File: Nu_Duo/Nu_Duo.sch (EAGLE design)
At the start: 11 parts, among them P1 XR_PREAMP, P2 XR_PREAMP, SW1 TDS08

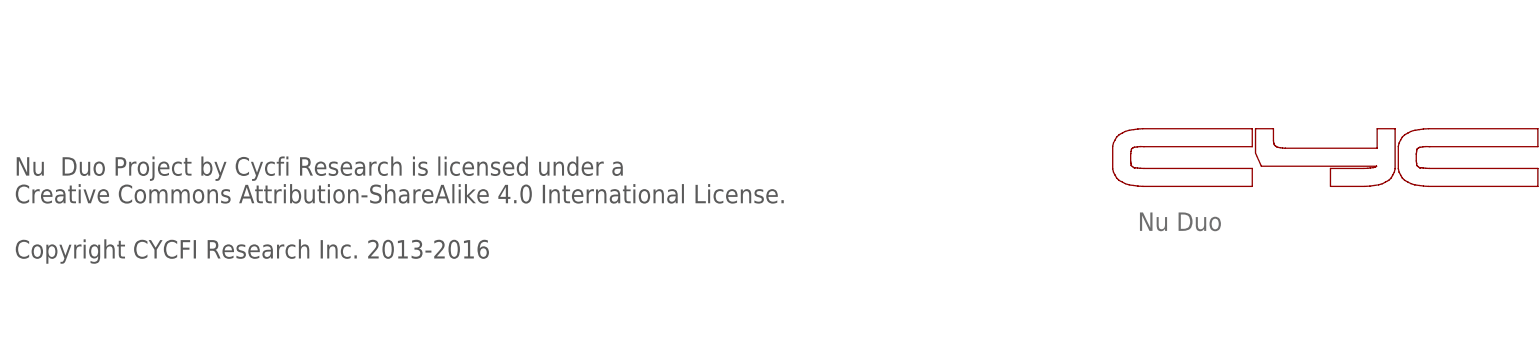
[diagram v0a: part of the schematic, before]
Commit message: *update license date
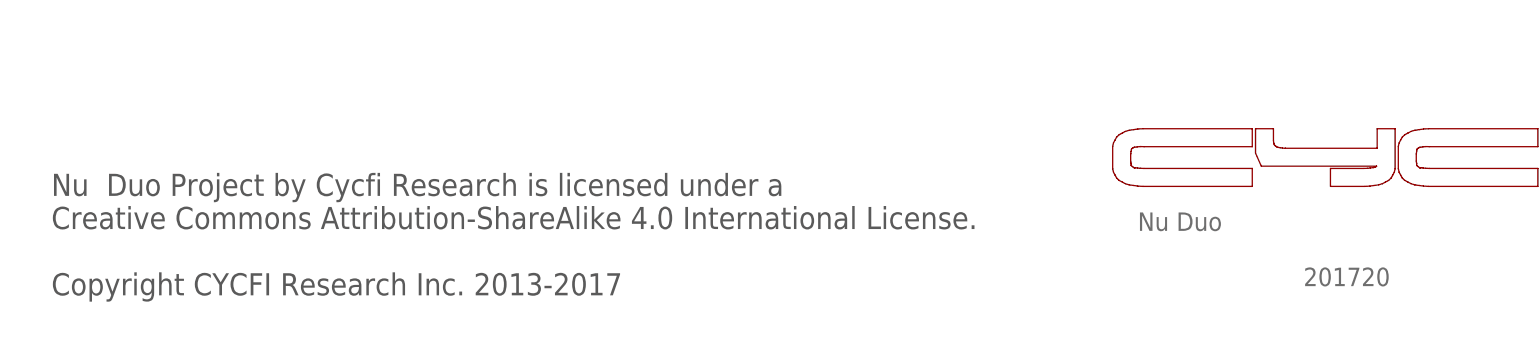
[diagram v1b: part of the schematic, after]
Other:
- note added: "201720"
- note added: "Nu Duo Project by Cycfi Research is licensed under a Creative Commons Attribution-ShareAlike 4.0 International License. Copyright CYCFI Research Inc. 2013-2017"
- note removed: "Nu Duo Project by Cycfi Research is licensed under a Creative Commons Attribution-ShareAlike 4.0 International License. Copyright CYCFI Research Inc. 2013-2016"
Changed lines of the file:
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@@
 <text x="208.915" y="113.665" size="1.778" layer="95">VCC</text>
 <text x="238.76" y="6.35" size="2.54" layer="95">2.0</text>
-<text x="7.62" y="15.24" size="2.54" layer="97">Nu  Duo Project by Cycfi Research is licensed under a
+<text x="12.7" y="10.16" size="3.048" layer="97">Nu  Duo Project by Cycfi Research is licensed under a
 Creative Commons Attribution-ShareAlike 4.0 International License.
-Copyright CYCFI Research Inc. 2013-2016</text>
+Copyright CYCFI Research Inc. 2013-2017</text>
+<text x="185.42" y="11.43" size="2.54" layer="95">201720</text>
 </plain>
 <instances>
